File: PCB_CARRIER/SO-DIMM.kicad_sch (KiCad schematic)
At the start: 1 part, among them J1 SODIMM-260_Split

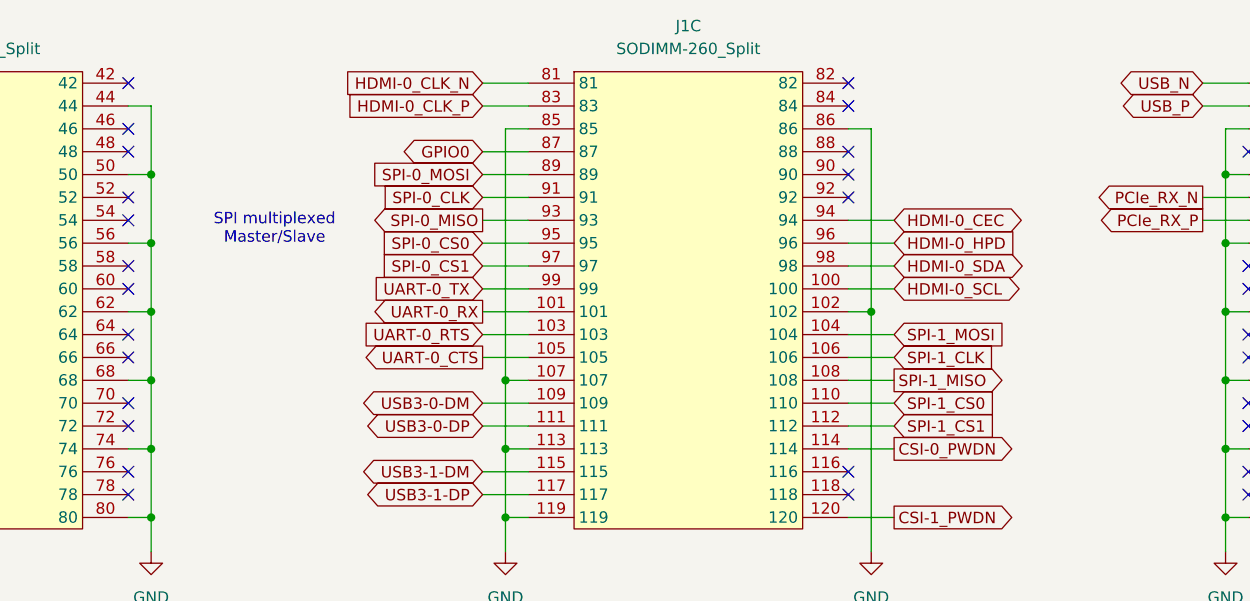
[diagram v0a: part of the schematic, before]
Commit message: fixed SPI, mislabelled some stuff
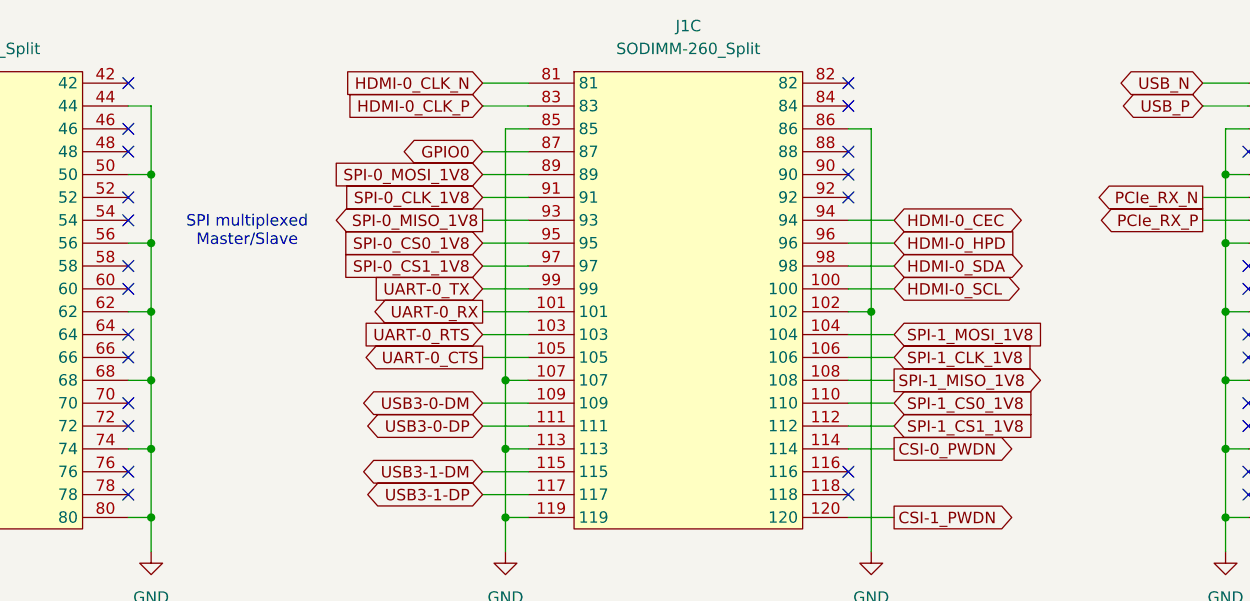
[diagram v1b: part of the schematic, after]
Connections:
- net SPI-0_CLK renamed SPI-0_CLK_1V8
- net SPI-0_CS0 renamed SPI-0_CS0_1V8
- net SPI-0_CS1 renamed SPI-0_CS1_1V8
- net SPI-0_MISO renamed SPI-0_MISO_1V8
- net SPI-0_MOSI renamed SPI-0_MOSI_1V8
- net SPI-1_CLK renamed SPI-1_CLK_1V8
- net SPI-1_CS0 renamed SPI-1_CS0_1V8
- net SPI-1_CS1 renamed SPI-1_CS1_1V8
- net SPI-1_MISO renamed SPI-1_MISO_1V8
- net SPI-1_MOSI renamed SPI-1_MOSI_1V8
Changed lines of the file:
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@@
 	(text "SPI multiplexed\nMaster/Slave"
 		(exclude_from_sim no)
-		(at 208.026 92.456 0)
+		(at 204.978 92.71 0)
 		(effects
 			(font
@@
 		)
 	)
-	(global_label "SPI-0_CS0"
+	(global_label "SPI-0_CS0_1V8"
 		(shape input)
 		(at 231.14 93.98 180)
@@
 		)
 		(property "Intersheetrefs" "${INTERSHEET_REFS}"
-			(at 217.5369 93.98 0)
+			(at 213.0617 93.98 0)
 			(effects
 				(font
@@
 		)
 	)
-	(global_label "SPI-1_CLK"
+	(global_label "SPI-1_CLK_1V8"
 		(shape input)
 		(at 276.86 106.68 0)
@@
 		)
 		(property "Intersheetrefs" "${INTERSHEET_REFS}"
-			(at 290.3422 106.68 0)
+			(at 294.8174 106.68 0)
 			(effects
 				(font
@@
 		)
 	)
-	(global_label "SPI-0_CS1"
+	(global_label "SPI-0_CS1_1V8"
 		(shape input)
 		(at 231.14 96.52 180)
@@
 		)
 		(property "Intersheetrefs" "${INTERSHEET_REFS}"
-			(at 217.5369 96.52 0)
+			(at 213.0617 96.52 0)
 			(effects
 				(font
@@
 		)
 	)
-	(global_label "SPI-1_CS0"
+	(global_label "SPI-1_CS0_1V8"
 		(shape input)
 		(at 276.86 111.76 0)
@@
 		)
 		(property "Intersheetrefs" "${INTERSHEET_REFS}"
-			(at 290.4631 111.76 0)
+			(at 294.9383 111.76 0)
 			(effects
 				(font
@@
 		)
 	)
-	(global_label "SPI-0_MOSI"
+	(global_label "SPI-0_MOSI_1V8"
 		(shape input)
 		(at 231.14 86.36 180)
@@
 		)
 		(property "Intersheetrefs" "${INTERSHEET_REFS}"
-			(at 216.6297 86.36 0)
+			(at 212.1545 86.36 0)
 			(effects
 				(font
@@
 		)
 	)
-	(global_label "SPI-1_MISO"
+	(global_label "SPI-1_MISO_1V8"
 		(shape output)
 		(at 276.86 109.22 0)
@@
 		)
 		(property "Intersheetrefs" "${INTERSHEET_REFS}"
-			(at 291.3703 109.22 0)
+			(at 295.8455 109.22 0)
 			(effects
 				(font
@@
 		)
 	)
-	(global_label "SPI-1_MOSI"
+	(global_label "SPI-1_MOSI_1V8"
 		(shape input)
 		(at 276.86 104.14 0)
@@
 		)
 		(property "Intersheetrefs" "${INTERSHEET_REFS}"
-			(at 291.3703 104.14 0)
+			(at 295.8455 104.14 0)
 			(effects
 				(font
@@
 		)
 	)
-	(global_label "SPI-0_CLK"
+	(global_label "SPI-0_CLK_1V8"
 		(shape input)
 		(at 231.14 88.9 180)
@@
 		)
 		(property "Intersheetrefs" "${INTERSHEET_REFS}"
-			(at 217.6578 88.9 0)
+			(at 213.1826 88.9 0)
 			(effects
 				(font
@@
 		)
 	)
-	(global_label "SPI-0_MISO"
+	(global_label "SPI-0_MISO_1V8"
 		(shape output)
 		(at 231.14 91.44 180)
@@
 		)
 		(property "Intersheetrefs" "${INTERSHEET_REFS}"
-			(at 216.6297 91.44 0)
+			(at 212.1545 91.44 0)
 			(effects
 				(font
@@
 		)
 	)
-	(global_label "SPI-1_CS1"
+	(global_label "SPI-1_CS1_1V8"
 		(shape input)
 		(at 276.86 114.3 0)
@@
 		)
 		(property "Intersheetrefs" "${INTERSHEET_REFS}"
-			(at 290.4631 114.3 0)
+			(at 294.9383 114.3 0)
 			(effects
 				(font

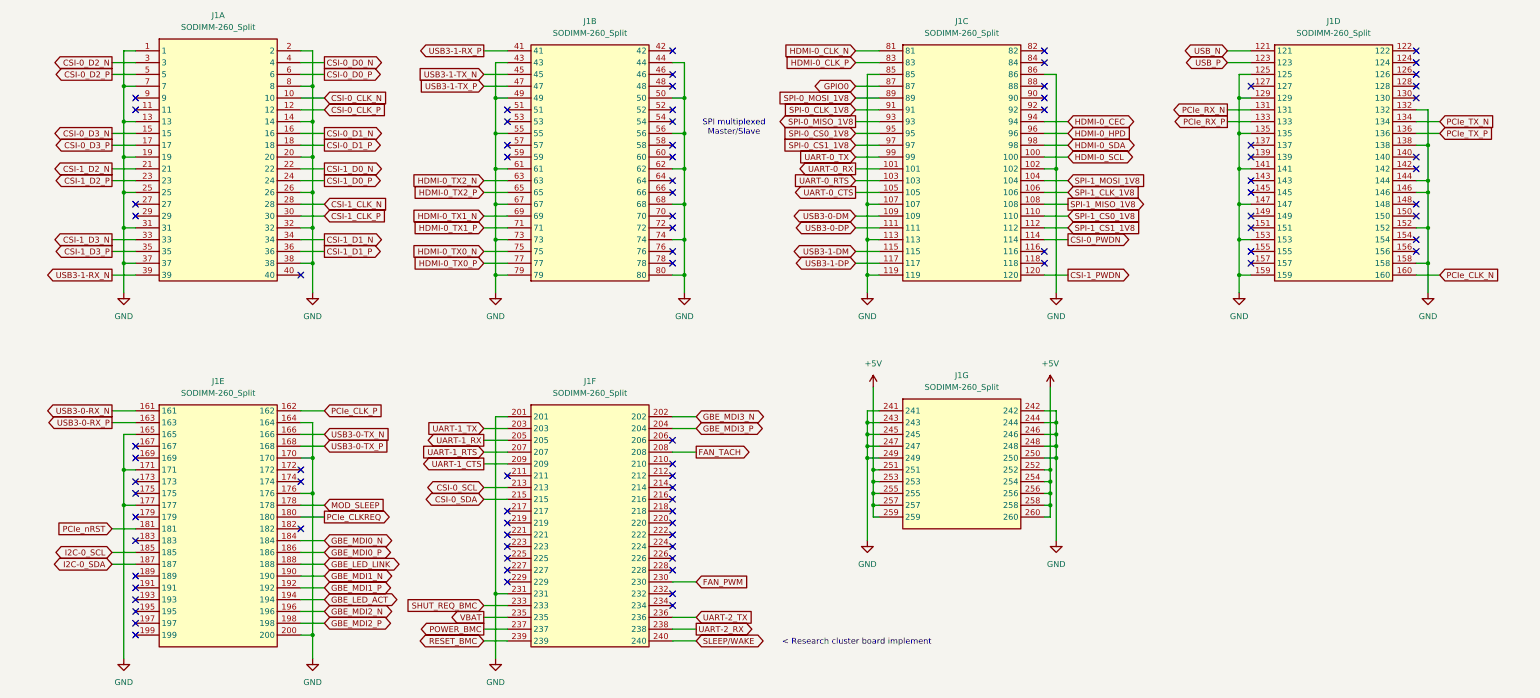
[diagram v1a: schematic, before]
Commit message: re-naming all UART signals for shifting preparation
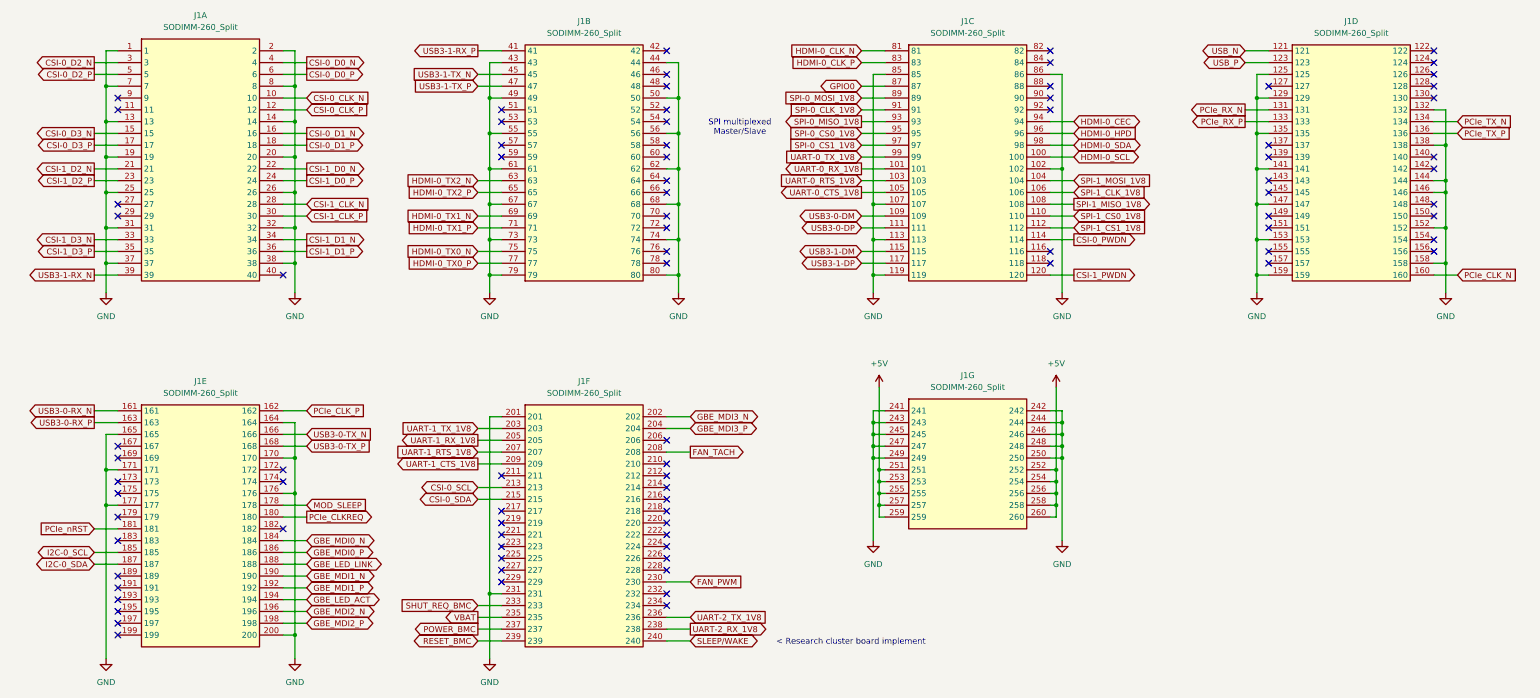
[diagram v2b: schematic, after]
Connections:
- net UART-0_CTS renamed UART-0_CTS_1V8
- net UART-0_RTS renamed UART-0_RTS_1V8
- net UART-0_RX renamed UART-0_RX_1V8
- net UART-0_TX renamed UART-0_TX_1V8
- net UART-1_CTS renamed UART-1_CTS_1V8
- net UART-1_RTS renamed UART-1_RTS_1V8
- net UART-1_RX renamed UART-1_RX_1V8
- net UART-1_TX renamed UART-1_TX_1V8
- net UART-2_RX renamed UART-2_RX_1V8
- net UART-2_TX renamed UART-2_TX_1V8
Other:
- moved on the sheet: J1A, J1B, J1C, J1D, J1E, J1F, J1G
